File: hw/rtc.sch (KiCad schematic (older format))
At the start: 3 parts

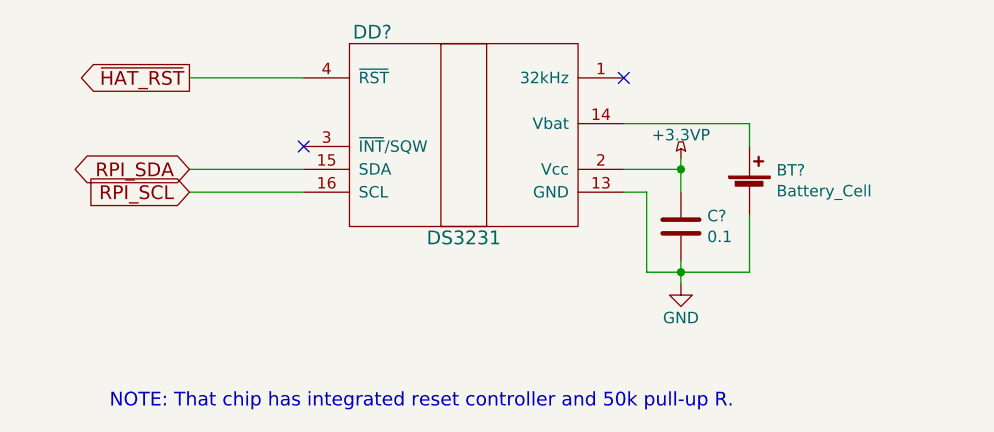
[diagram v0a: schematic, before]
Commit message: hw: start stm page
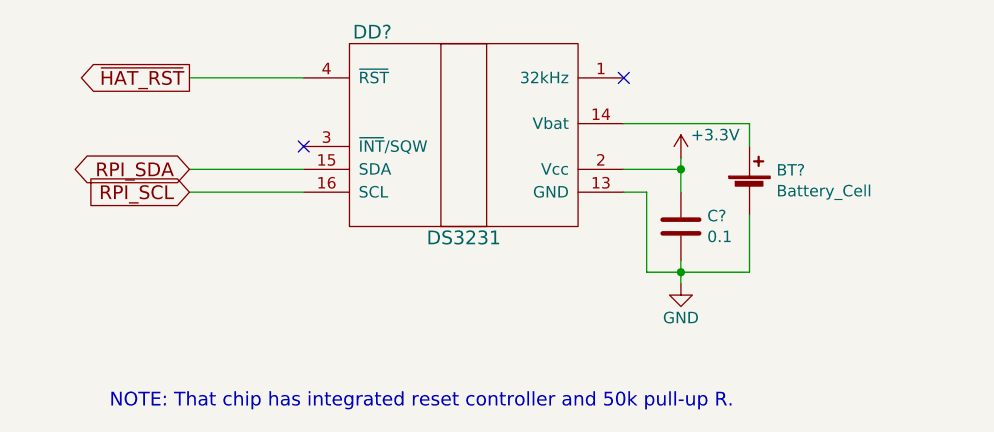
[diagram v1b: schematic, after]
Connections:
- net +3.3VP renamed +3V3
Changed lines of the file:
@@
-	1    0    0    -1
-$EndComp
-$Comp
-L power:+3.3VP #PWR?
-U 1 1 5AB3BD26
-P 5350 5100
-F 0 "#PWR?" H 5500 5050 50  0001 C CNN
-F 1 "+3.3VP" H 5350 5200 50  0000 C CNN
-F 2 "" H 5350 5100 50  0001 C CNN
-F 3 "" H 5350 5100 50  0001 C CNN
-	1    5350 5100
 	1    0    0    -1
 $EndComp
@@
 	1    0    0    -1
 $EndComp
+$Comp
+L power:+3.3V #PWR?
+U 1 1 5AC432E2
+P 5350 5100
+F 0 "#PWR?" H 5350 4950 50  0001 C CNN
+F 1 "+3.3V" H 5500 5200 50  0000 C CNN
+F 2 "" H 5350 5100 50  0001 C CNN
+F 3 "" H 5350 5100 50  0001 C CNN
+	1    5350 5100
+	1    0    0    -1
+$EndComp

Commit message: hw: update libs
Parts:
- DD?: symbol ic:DS3231 -> hat-ic:DS3231
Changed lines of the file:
@@
 $EndDescr
 $Comp
-L ic:DS3231 DD?
+L hat-ic:DS3231 DD?
 U 1 1 5AB3B4DF
 P 4400 5000

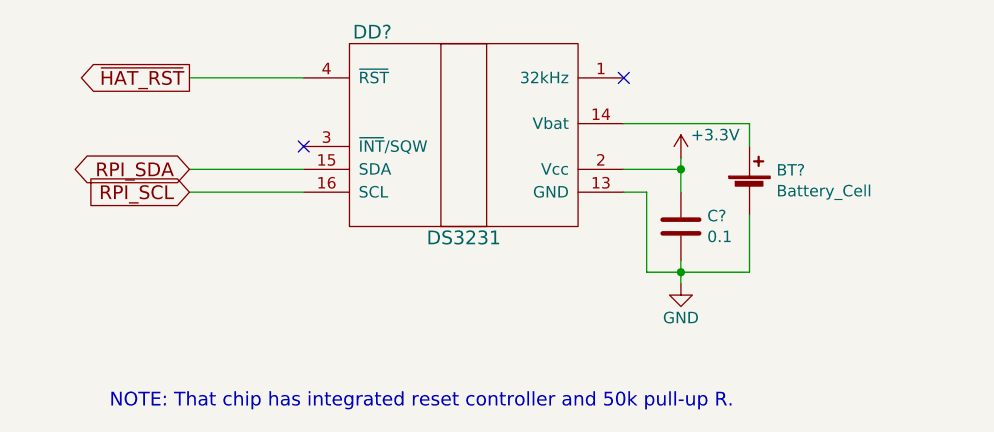
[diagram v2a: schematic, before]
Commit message: hw: sch ready
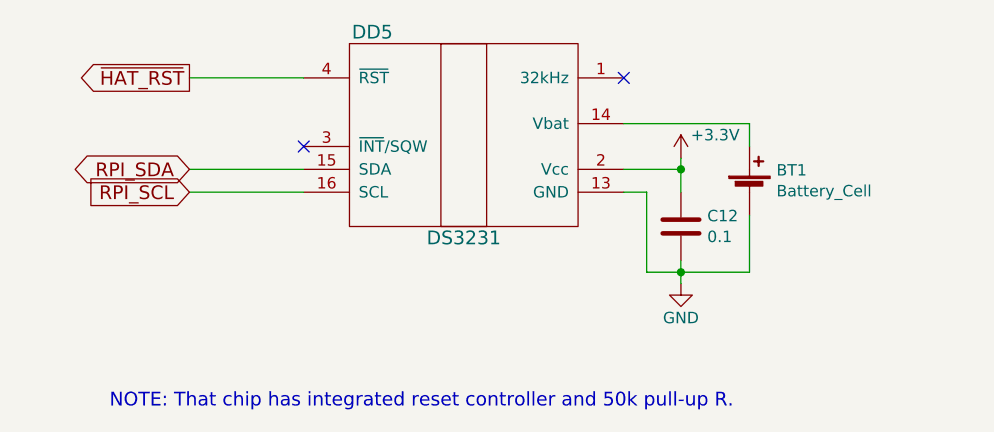
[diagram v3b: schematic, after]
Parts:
- gave numbers to parts that had none: 3
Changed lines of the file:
@@
 $EndDescr
 $Comp
-L hat-ic:DS3231 DD?
+L hat-ic:DS3231 DD5
 U 1 1 5AB3B4DF
 P 4400 5000
-F 0 "DD?" H 4000 5450 60  0000 C CNN
+F 0 "DD5" H 4000 5450 60  0000 C CNN
 F 1 "DS3231" H 4400 4550 60  0000 C CNN
 F 2 "Housings_SOIC:SOIC-16W_7.5x10.3mm_Pitch1.27mm" H 4400 5050 60  0001 C CNN
@@
 $EndComp
 $Comp
-L power:GND #PWR?
+L power:GND #PWR048
 U 1 1 5AB3BD10
 P 5350 5650
-F 0 "#PWR?" H 5350 5400 50  0001 C CNN
+F 0 "#PWR048" H 5350 5400 50  0001 C CNN
 F 1 "GND" H 5350 5500 50  0000 C CNN
 F 2 "" H 5350 5650 50  0001 C CNN
@@
 	5350 5150 5350 5250
 $Comp
-L Device:Battery_Cell BT?
+L Device:Battery_Cell BT1
 U 1 1 5AC0D5A2
 P 5650 5250
-F 0 "BT?" H 5768 5346 50  0000 L CNN
+F 0 "BT1" H 5768 5346 50  0000 L CNN
 F 1 "Battery_Cell" H 5768 5255 50  0000 L CNN
 F 2 "" V 5650 5310 50  0001 C CNN
@@
 $EndComp
 $Comp
-L Device:C C?
+L Device:C C12
 U 1 1 5AC0D763
 P 5350 5400
-F 0 "C?" H 5465 5446 50  0000 L CNN
+F 0 "C12" H 5465 5446 50  0000 L CNN
 F 1 "0.1" H 5465 5355 50  0000 L CNN
 F 2 "" H 5388 5250 50  0001 C CNN
@@
 $EndComp
 $Comp
-L power:+3.3V #PWR?
+L power:+3.3V #PWR047
 U 1 1 5AC432E2
 P 5350 5100
-F 0 "#PWR?" H 5350 4950 50  0001 C CNN
+F 0 "#PWR047" H 5350 4950 50  0001 C CNN
 F 1 "+3.3V" H 5500 5200 50  0000 C CNN
 F 2 "" H 5350 5100 50  0001 C CNN
